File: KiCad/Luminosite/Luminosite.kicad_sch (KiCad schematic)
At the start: 12 parts, among them J1 Conn_01x03, U1 MCP6022

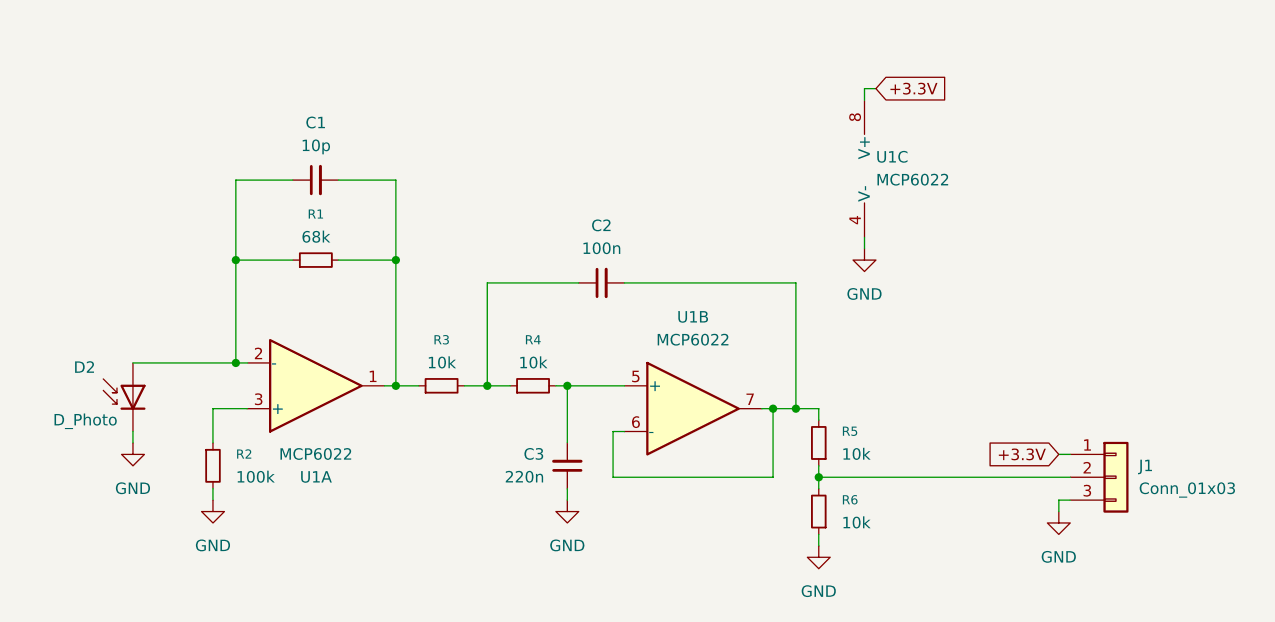
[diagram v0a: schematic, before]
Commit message: Capteur de température
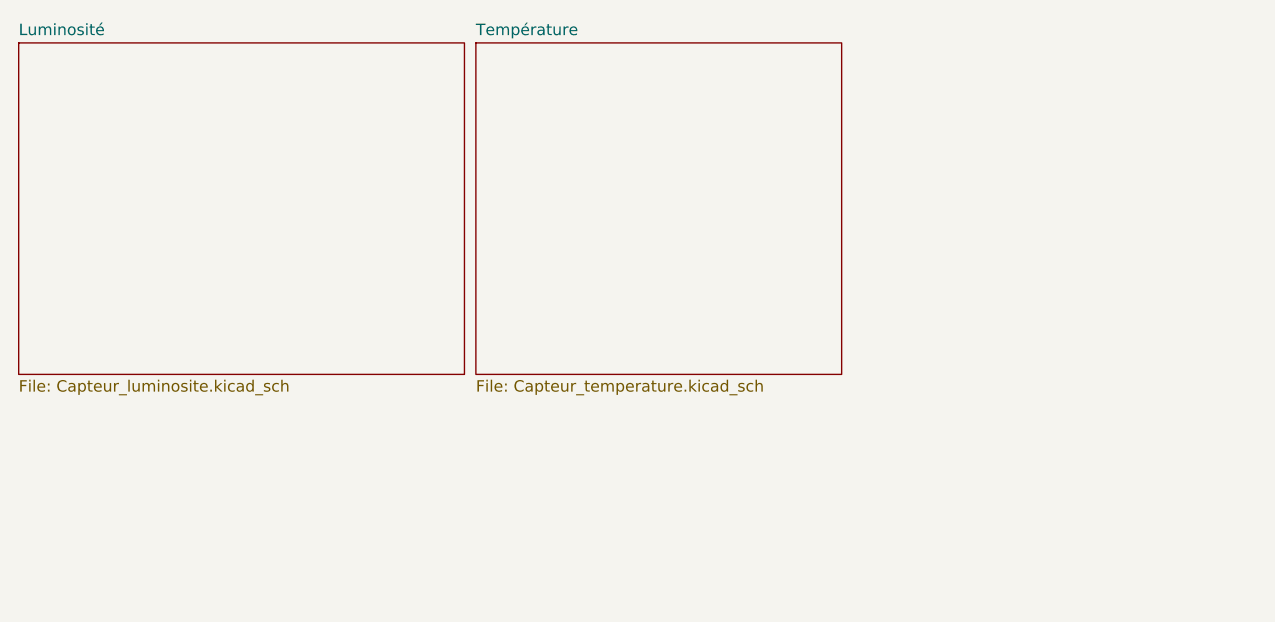
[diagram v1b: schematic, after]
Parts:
- removed C1: 10p, symbol Device:C_Small
- removed C2: 100n, symbol Device:C_Small
- removed C3: 220n, symbol Device:C_Small
- removed D2: D_Photo, symbol Device:D_Photo
- removed J1: Conn_01x03, symbol Connector_Generic:Conn_01x03
- removed R1: 68k, symbol Device:R_Small
- removed R2: 100k, symbol Device:R_Small
- removed R3, R4, R5, R6: 10k, symbol Device:R_Small
- removed U1: MCP6022, symbol Amplifier_Operational:MCP6022
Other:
- added sheet Luminosité (Capteur_luminosite.kicad_sch)
- added sheet Température (Capteur_temperature.kicad_sch)
